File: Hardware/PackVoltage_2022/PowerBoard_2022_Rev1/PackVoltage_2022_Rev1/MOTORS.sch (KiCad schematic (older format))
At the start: 63 parts

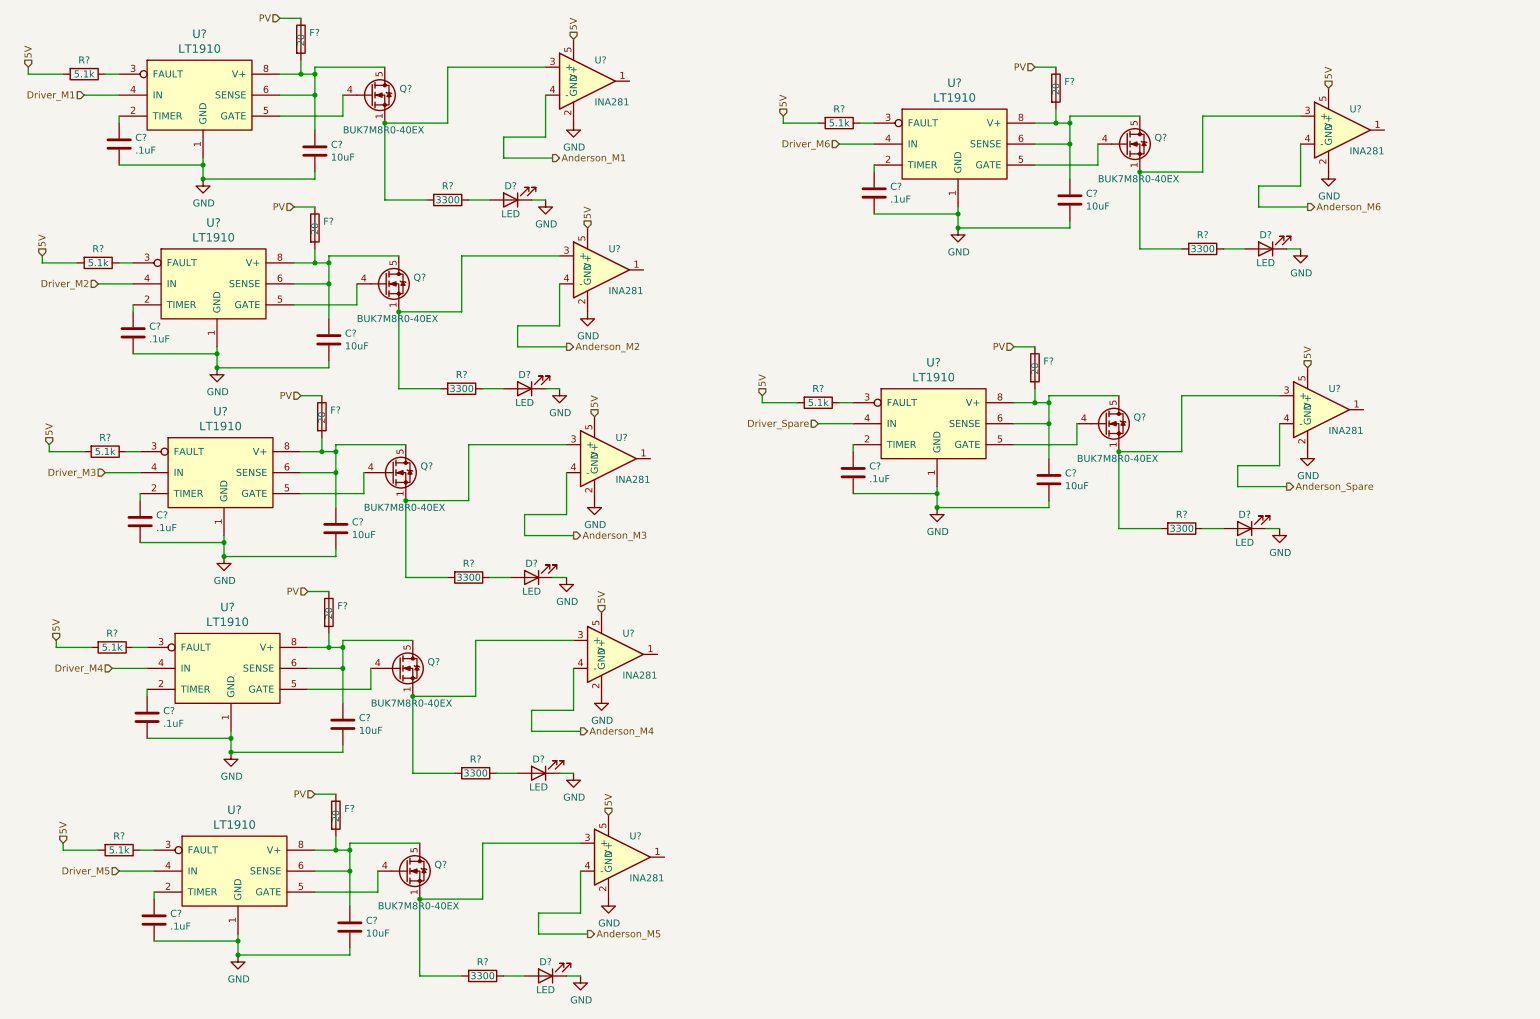
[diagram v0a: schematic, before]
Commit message: added andersons
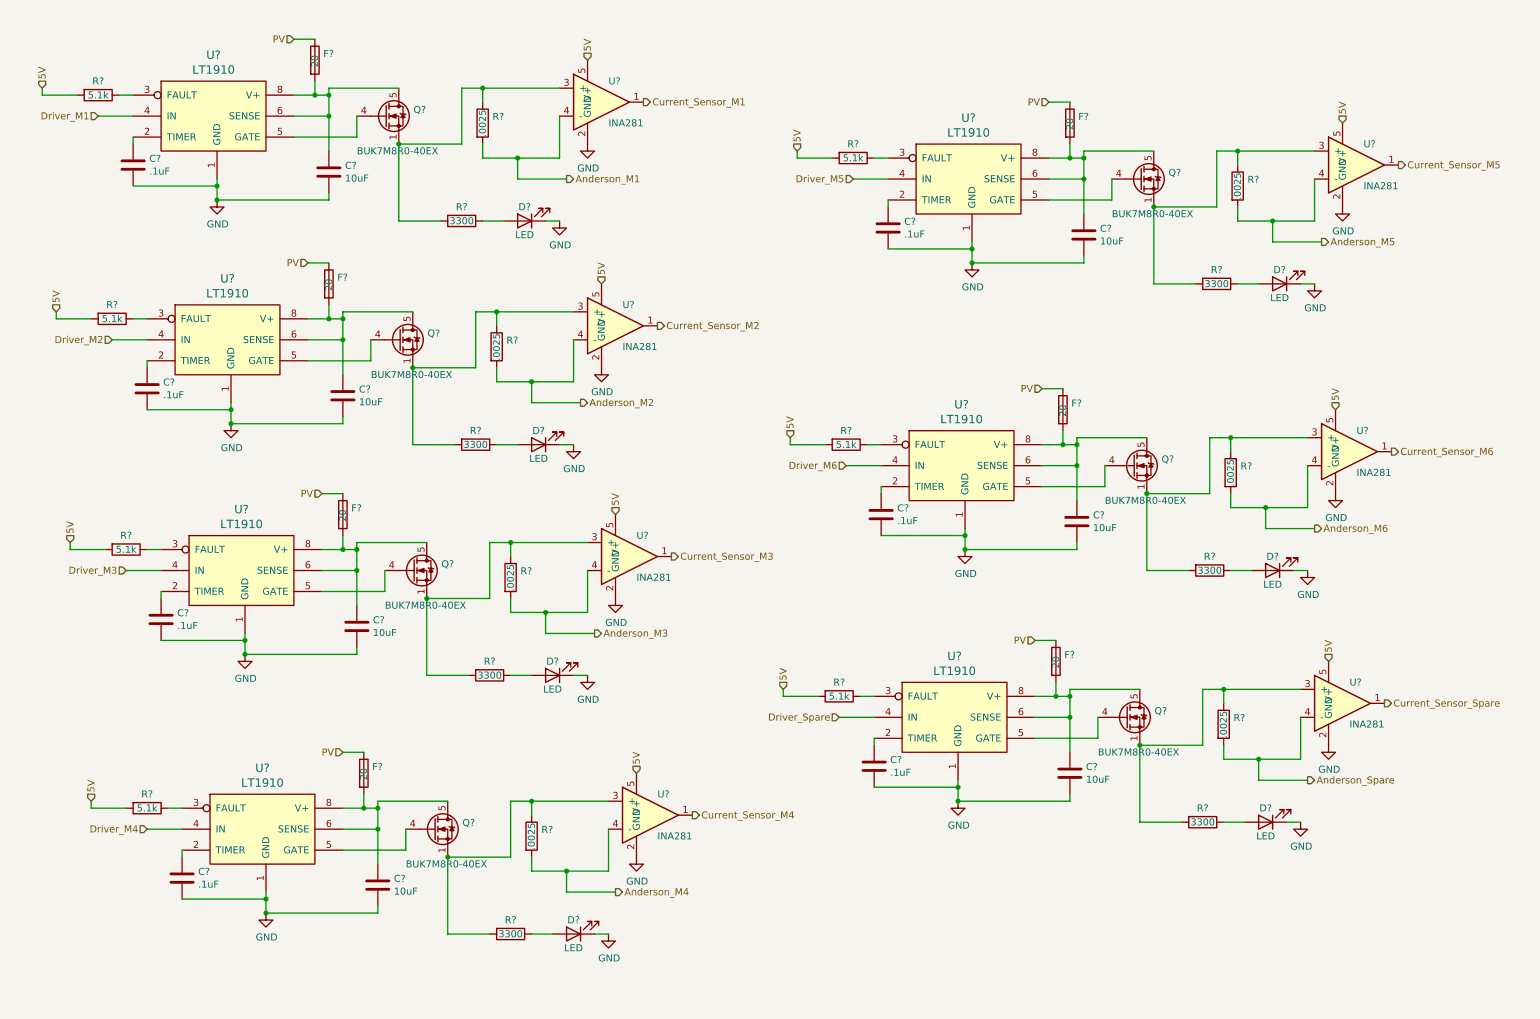
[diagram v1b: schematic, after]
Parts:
- removed C? (x7): .1uF, symbol Device:C
- removed C? (x7): 10uF, symbol Device:C
- removed D? (x7): LED, symbol Device:LED
- removed F? (x7): 20, symbol Device:Fuse
- removed Q? (x7): BUK7M8R0-40EX, Package_TO_SOT_SMD:LFPAK33, symbol Transistor_FET:BUK7M8R0-40EX
- removed R? (x7): 5.1k, symbol Device:R
- removed R? (x7): 3300, symbol Device:R
- removed U? (x7): LT1910, symbol MRDT_ICs:LT1910
- removed U? (x7): INA281, Package_TO_SOT_SMD:SOT-23-5, symbol MRDT_ICs:INA281
- added C? (x7): .1uF, symbol Device:C
- added C? (x7): 10uF, symbol Device:C
- added D? (x7): LED, symbol Device:LED
- added F? (x7): 20, symbol Device:Fuse
- added Q? (x7): BUK7M8R0-40EX, Package_TO_SOT_SMD:LFPAK33, symbol Transistor_FET:BUK7M8R0-40EX
- added R? (x7): 5.1k, symbol Device:R
- added R? (x7): 3300, symbol Device:R
- added R? (x7): .0025, symbol Device:R
- added U? (x7): LT1910, symbol MRDT_ICs:LT1910
- added U? (x7): INA281, Package_TO_SOT_SMD:SOT-23-5, symbol MRDT_ICs:INA281
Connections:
- net 5V: now also R?.2, R?.2, R?.2, R?.2, R?.2, R?.2, R?.2, U?.5 (V+), U?.5 (V+), U?.5 (V+), U?.5 (V+), U?.5 (V+), U?.5 (V+), U?.5 (V+)
- net Anderson_M1: now also R?.2, U?.4 (-)
- net Anderson_M2: now also R?.2, U?.4 (-)
- net Anderson_M3: now also R?.2, U?.4 (-)
- net Anderson_M4: now also R?.2, U?.4 (-)
- net Anderson_M5: now also R?.2, U?.4 (-)
- net Anderson_M6: now also R?.2, U?.4 (-)
- net Anderson_Spare: now also R?.2, U?.4 (-)
- net Driver_M1: now also U?.4 (IN)
- net Driver_M2: now also U?.4 (IN)
- net Driver_M3: now also U?.4 (IN)
- net Driver_M4: now also U?.4 (IN)
- net Driver_M5: now also U?.4 (IN)
- net Driver_M6: now also U?.4 (IN)
- net Driver_Spare: now also U?.4 (IN)
- net GND: now also C?.2, C?.2, C?.2, C?.2, C?.2, C?.2, C?.2, C?.2, C?.2, C?.2, C?.2, C?.2, C?.2, C?.2, D?.1 (K), D?.1 (K), D?.1 (K), D?.1 (K), D?.1 (K), D?.1 (K), D?.1 (K), U?.1 (GND), U?.1 (GND), U?.1 (GND), U?.1 (GND), U?.1 (GND), U?.1 (GND), U?.1 (GND), U?.2 (GND), U?.2 (GND), U?.2 (GND), U?.2 (GND), U?.2 (GND), U?.2 (GND), U?.2 (GND)
- net PV: now also F?.1, F?.1, F?.1, F?.1, F?.1, F?.1, F?.1
- new net: R?.1, U?.3 (FAULT) (x7)
- new net: C?.1, U?.2 (TIMER) (x7)
- new net: Q?.4 (G), U?.5 (GATE) (x7)
- new net: C?.1, F?.2, Q?.5 (D), U?.6 (SENSE), U?.8 (V+) (x7)
- new net: Q?.1 (S), Q?.2 (S), Q?.3 (S), R?.1, R?.2, U?.3 (+) (x7)
- new net: D?.2 (A), R?.1 (x7)
- new net Current_Sensor_M1: U?.1
- new net Current_Sensor_M2: U?.1
- new net Current_Sensor_M3: U?.1
- new net Current_Sensor_M4: U?.1
- new net Current_Sensor_M5: U?.1
- new net Current_Sensor_M6: U?.1
- new net Current_Sensor_Spare: U?.1
